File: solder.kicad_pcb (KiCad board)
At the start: 2 copper layers, 41 x 36.6 mm, 6 parts

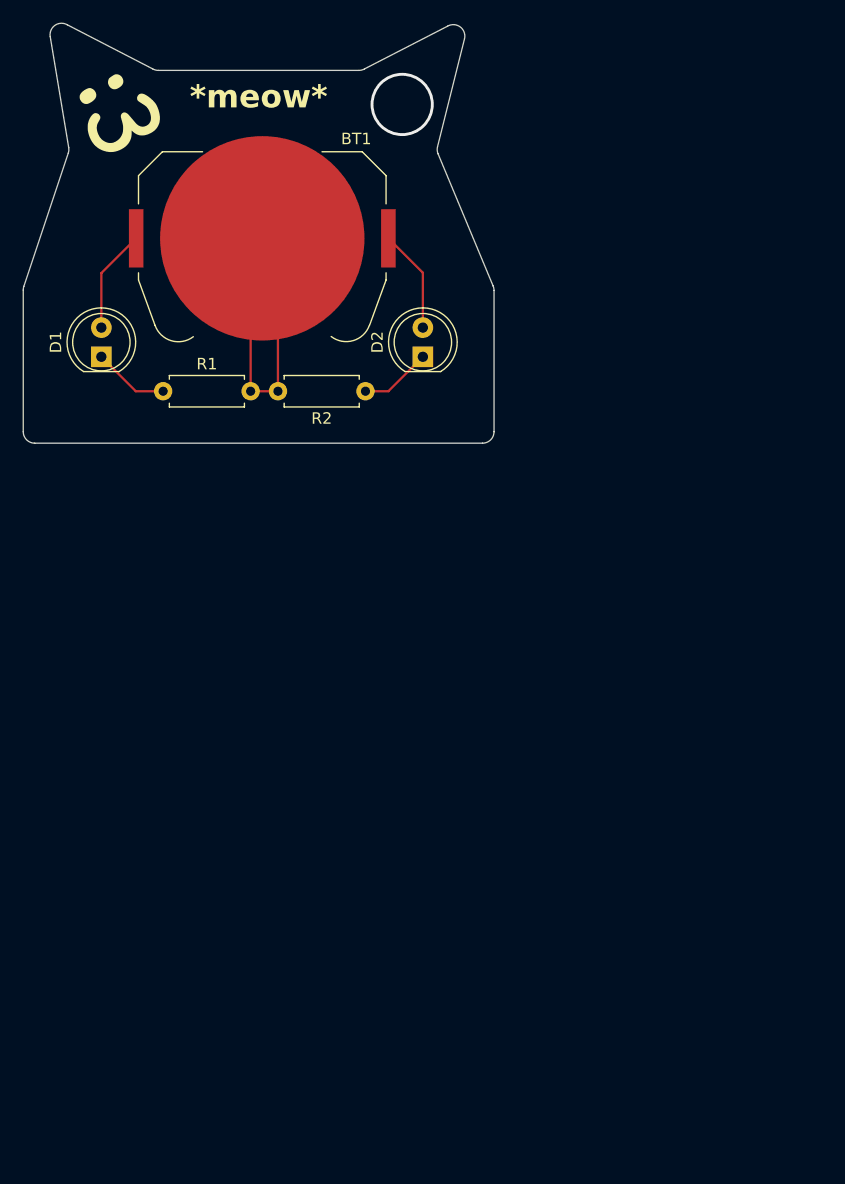
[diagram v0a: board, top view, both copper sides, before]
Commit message: update!!! made LEDs blink
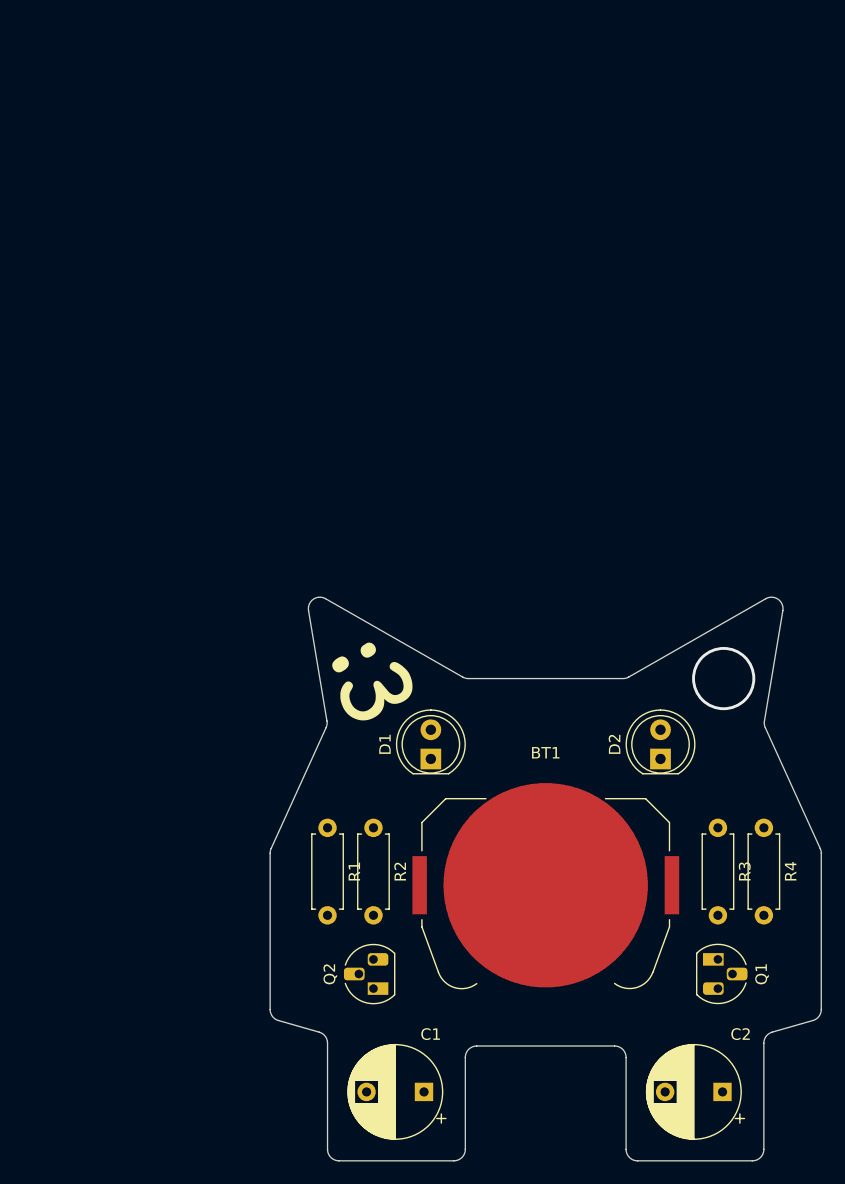
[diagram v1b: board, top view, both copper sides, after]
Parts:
- added C1: C, Capacitor_THT:CP_Radial_D8.0mm_P5.00mm, F.Cu at (114.4, 143.0)
- added C2: C, Capacitor_THT:CP_Radial_D8.0mm_P5.00mm, F.Cu at (140.4, 143.0)
- added Q1: NPN, Package_TO_SOT_THT:TO-92L_HandSolder, F.Cu at (140.0, 131.5)
- added Q2: NPN, Package_TO_SOT_THT:TO-92L_HandSolder, F.Cu at (110.0, 134.0)
- added R3: R, Resistor_THT:R_Axial_DIN0207_L6.3mm_D2.5mm_P7.62mm_Horizontal, F.Cu at (140.0, 120.0)
- added R4: R, Resistor_THT:R_Axial_DIN0207_L6.3mm_D2.5mm_P7.62mm_Horizontal, F.Cu at (144.0, 120.0)
- moved BT1 61.5 mm to (125.0, 125.0)
- moved G*** 54.2 mm to (110.0, 107.0)
- moved D1 45.3 mm to (115.0, 114.0)
- moved D2 40.7 mm to (135.0, 114.0)
- moved R1 40.6 mm to (106.0, 120.0), turned to -90 degrees
- moved R2 38.0 mm to (110.0, 120.0), turned to -90 degrees
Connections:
- R1 pad 1: Net-(D1-K) -> Net-(BT1-+)
- R1 pad 2: Net-(BT1--) -> Net-(D1-K)
- R2 pad 1: Net-(D2-K) -> Net-(BT1-+)
- R2 pad 2: Net-(BT1--) -> Net-(Q2-B)
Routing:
- net Net-(BT1--): track 30.0 -> 0.00 mm
- net Net-(BT1-+): track 18.1 -> 0.00 mm
- net Net-(D1-K): track 6.62 -> 0.00 mm
- net Net-(D2-K): track 6.24 -> 0.00 mm
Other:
- board size 41 x 36.6 mm -> 48 x 49.1 mm
- board text removed: "*meow*"
